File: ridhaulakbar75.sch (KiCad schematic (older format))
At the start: 184 parts, among them J1 SWD, J2 Ex_Bat, J3 Ex_USB, J4 RESET, J5 Underglow, Q1 AO3407, Q2 AO3407, SW1 Rotary_Encoder_Switch, U2 E73-2G4M08S1C-52840, U3 XC6220B331MR, U4 TP4054, Y1 32.768kHz

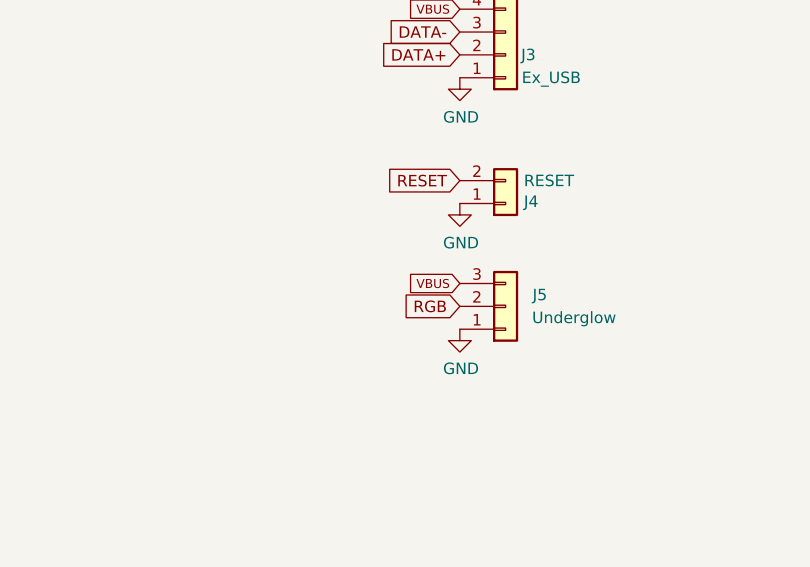
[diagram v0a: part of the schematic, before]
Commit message: final
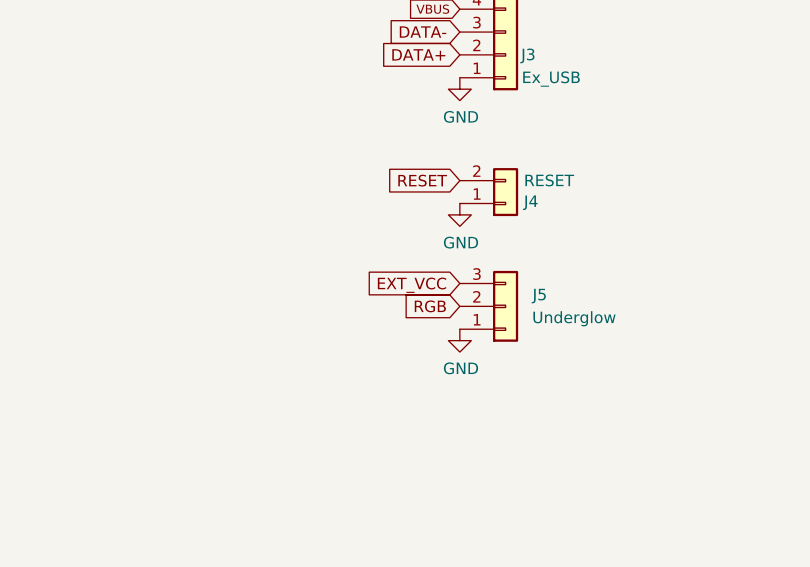
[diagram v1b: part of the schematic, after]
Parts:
- J5: footprint Connector_PinHeader_2.54mm:PinHeader_1x03_P2.54mm_Vertical -> Connector_PinHeader_2.00mm:PinHeader_1x03_P2.00mm_Vertical
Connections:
- net EXT_VCC: now also J5.3 (Pin_3)
- net VBUS: no longer J5.3 (Pin_3)
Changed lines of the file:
@@
 F 0 "J5" H 11600 5400 50  0000 C CNN
 F 1 "Underglow" H 11750 5500 50  0000 C CNN
-F 2 "Connector_PinHeader_2.54mm:PinHeader_1x03_P2.54mm_Vertical" H 11450 5450 50  0001 C CNN
+F 2 "Connector_PinHeader_2.00mm:PinHeader_1x03_P2.00mm_Vertical" H 11450 5450 50  0001 C CNN
 F 3 "~" H 11450 5450 50  0001 C CNN
 	1    11450 5450
@@
 	1    0    0    -1
 $EndComp
-Text GLabel 11250 5350 0    39   Input ~ 0
-VBUS
 Text GLabel 11250 5450 0    50   Input ~ 0
 RGB
 Text GLabel 1650 9750 0    50   Input ~ 0
 RGB
+Text GLabel 11250 5350 0    50   Input ~ 0
+EXT_VCC
 $EndSCHEMATC
